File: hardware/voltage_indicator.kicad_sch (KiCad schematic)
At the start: 15 parts, among them J1 HV+, J2 HV-, U2 LM211DT

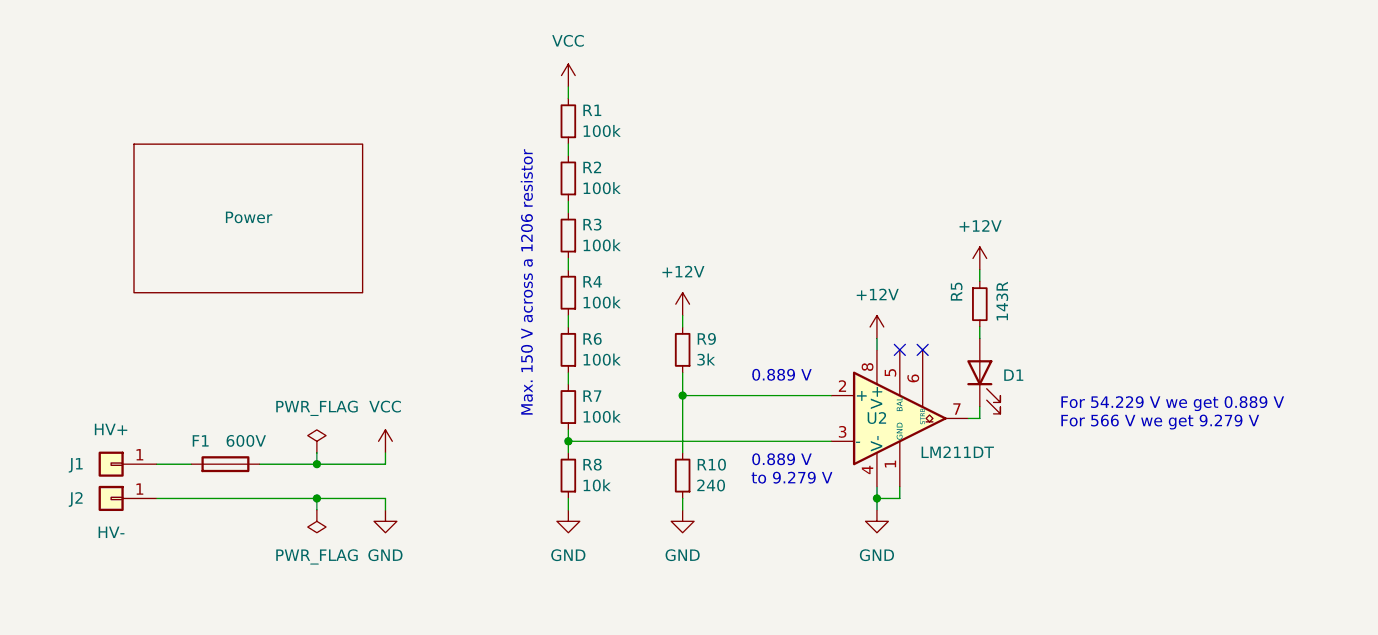
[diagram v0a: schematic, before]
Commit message: Improve the layout
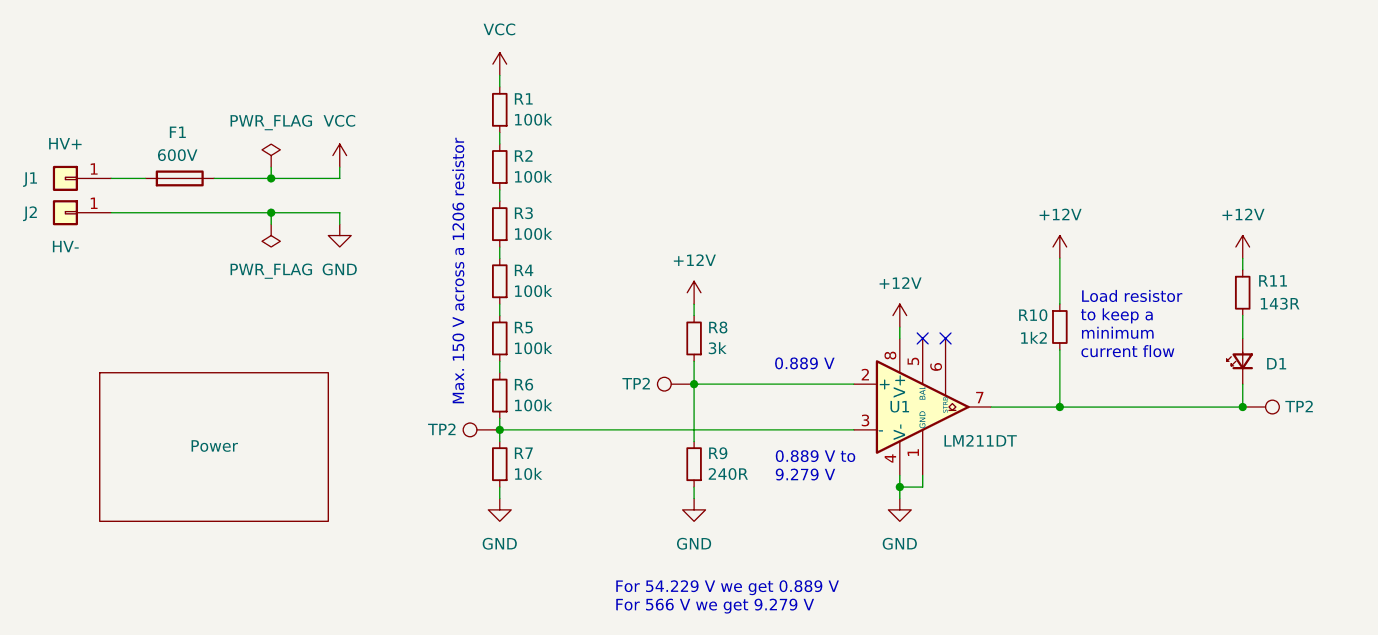
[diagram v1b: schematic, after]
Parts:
- added R10: 1k2, Resistor_SMD:R_0603_1608Metric, symbol Device:R_Small
- added TP2: LM_N, TestPoint:TestPoint_Pad_D1.0mm, symbol Connector:TestPoint
- added TP2: LM_OUT, TestPoint:TestPoint_Pad_D1.0mm, symbol Connector:TestPoint
- added TP2: LM_P, TestPoint:TestPoint_Pad_D1.0mm, symbol Connector:TestPoint
- D1: footprint LED_THT:LED_D5.0mm -> LED_THT:LED_Rectangular_W3.9mm_H1.9mm; symbol Device:LED -> Device:LED_Small
- F1: footprint vindicator:01020071Z-FUSE-CLIP -> Local_Library:FuseClip
- J1, J2: footprint Connector_Wire:SolderWire-0.5sqmm_1x01_D0.9mm_OD2.1mm_Relief -> Local_Library:SolderWire_Relief
- R9: renamed from R10; value 240 -> 240R
- renumbered R5 to R11, R6 to R5, R7 to R6, R8 to R7, R9 to R8, U2 to U1
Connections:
- net +12V: now also R10.1
- net at R6.1, R7.2, U1.3 (-): now also TP2.1
- net at R8.1, R9.2, U1.2 (+): now also TP2.1
- net at D1.1 (K), U1.7: now also R10.2, TP2.1
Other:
- note removed: "0.889 V to 9.279 V"
- note removed: "For 54.229 V we get 0.889 V For 566 V we get 9.279 V"
- company: (none) -> H. Fedarovich
- moved on the sheet: D1, F1, J1, J2, R1, R11, R2, R3, R4, R5, R6, R7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
